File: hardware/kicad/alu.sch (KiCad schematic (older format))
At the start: 6 parts

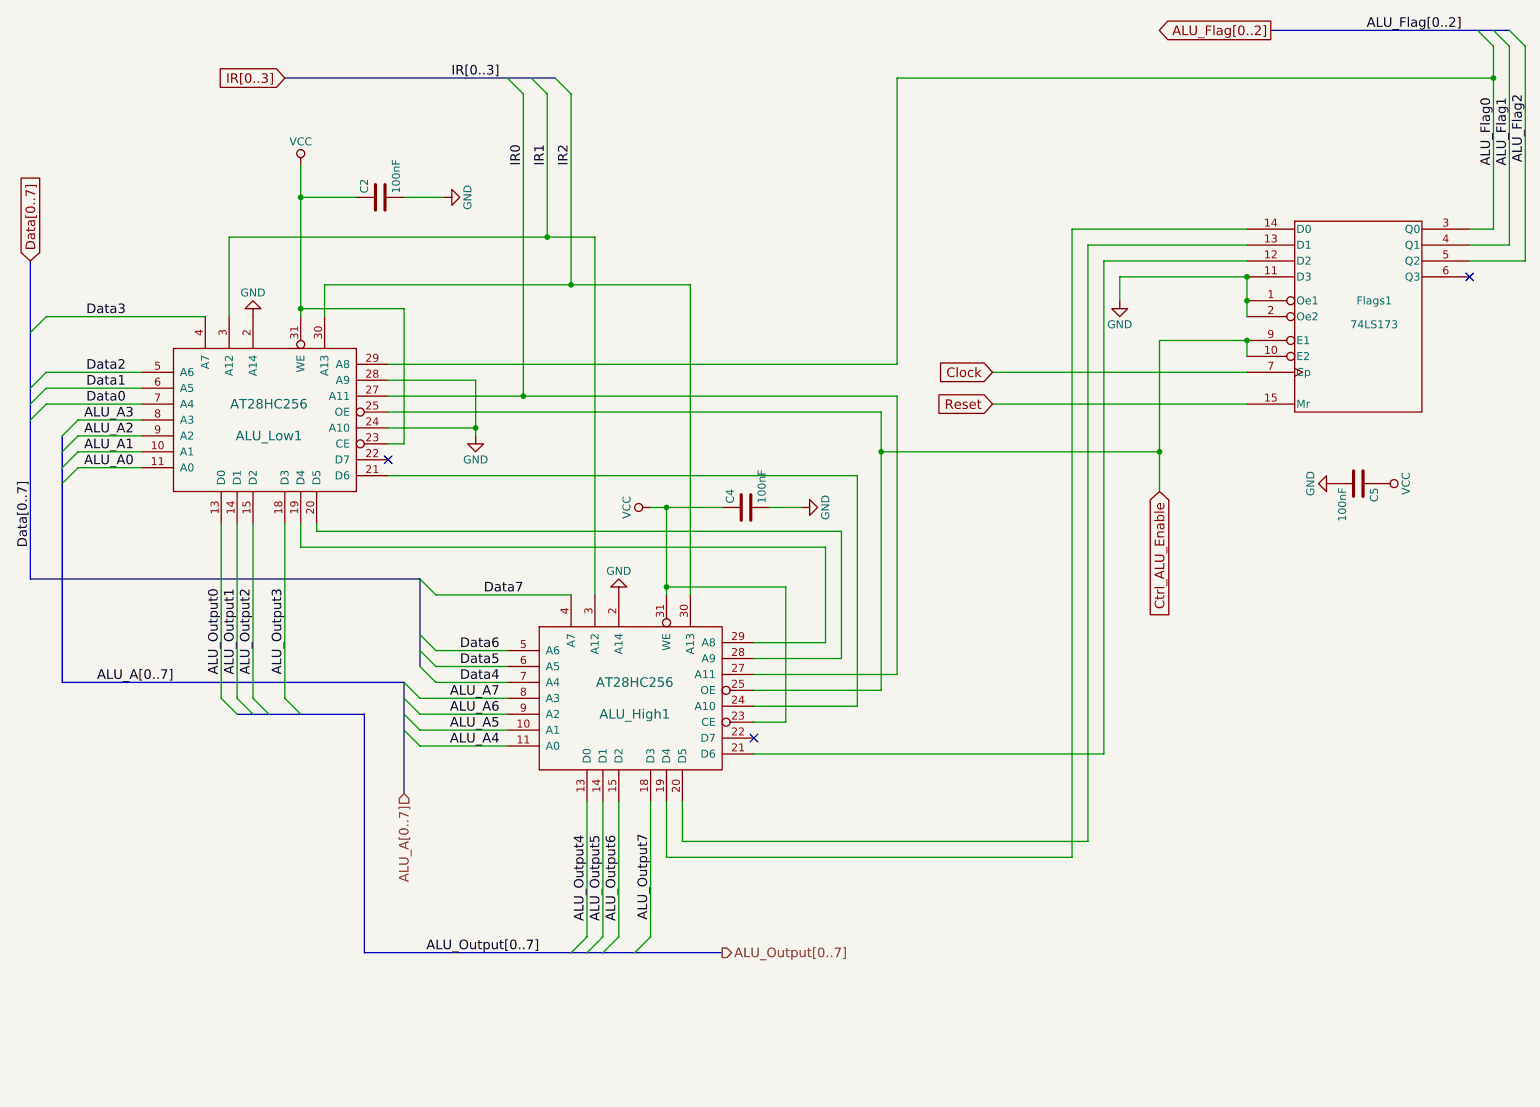
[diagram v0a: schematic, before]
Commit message: Just a backup.
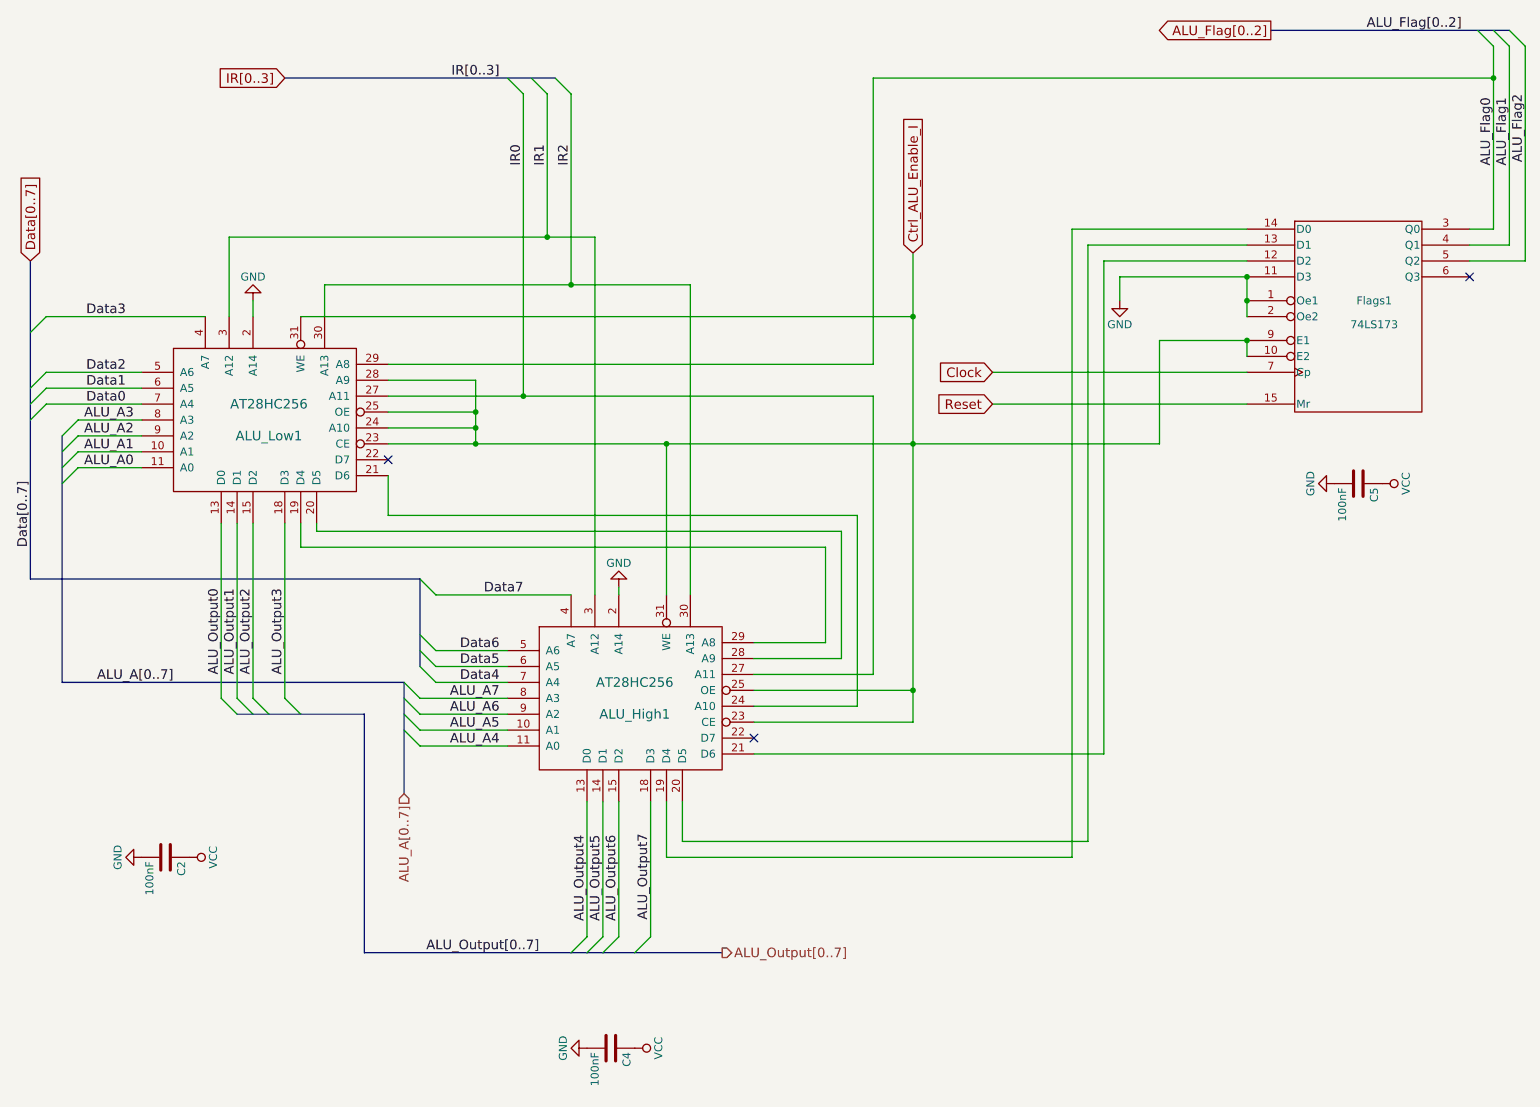
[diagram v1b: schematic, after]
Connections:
- net GND: no longer ALU_Low1.24 (A10), ALU_Low1.28 (A9)
- net VCC: no longer ALU_High1.23 (CE), ALU_High1.31 (WE), ALU_Low1.23 (CE), ALU_Low1.31 (WE)
- net Ctrl_ALU_Enable renamed Ctrl_ALU_Enable_I
- net Ctrl_ALU_Enable_I: now also ALU_High1.23 (CE), ALU_High1.31 (WE), ALU_Low1.23 (CE), ALU_Low1.24 (A10), ALU_Low1.28 (A9), ALU_Low1.31 (WE)
